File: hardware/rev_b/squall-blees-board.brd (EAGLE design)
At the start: 25.4 x 21 mm, 12 parts, among them J1 SQUALL_HEADER, J4 HIROSE-DF40C-10DP-0.4V, J5 HIROSE-DF40C-10DP-0.4V

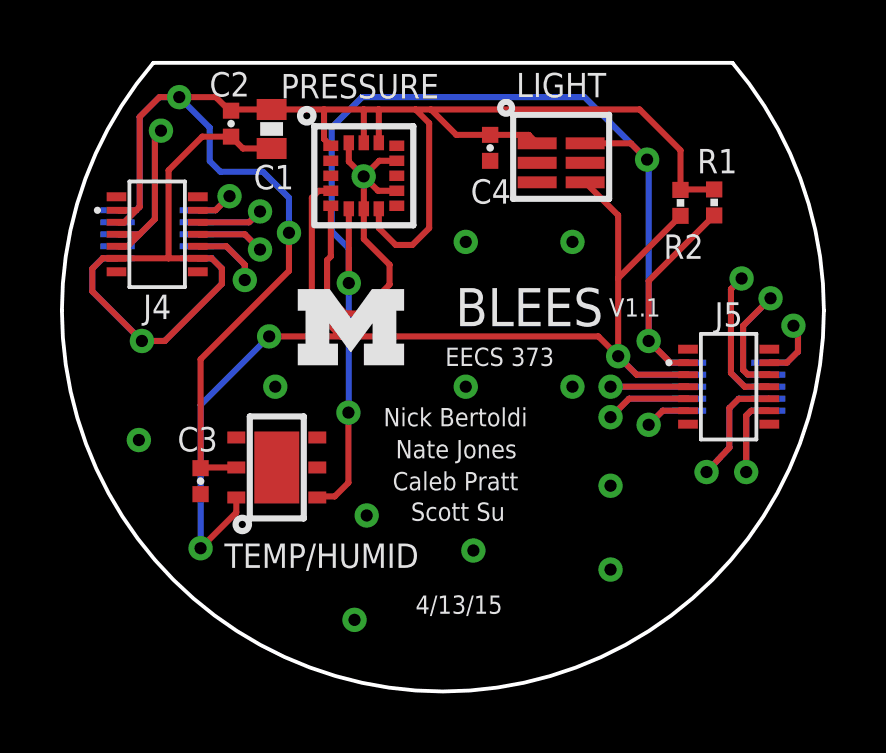
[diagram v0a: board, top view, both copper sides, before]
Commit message: Update rev_b, send it for fabrication
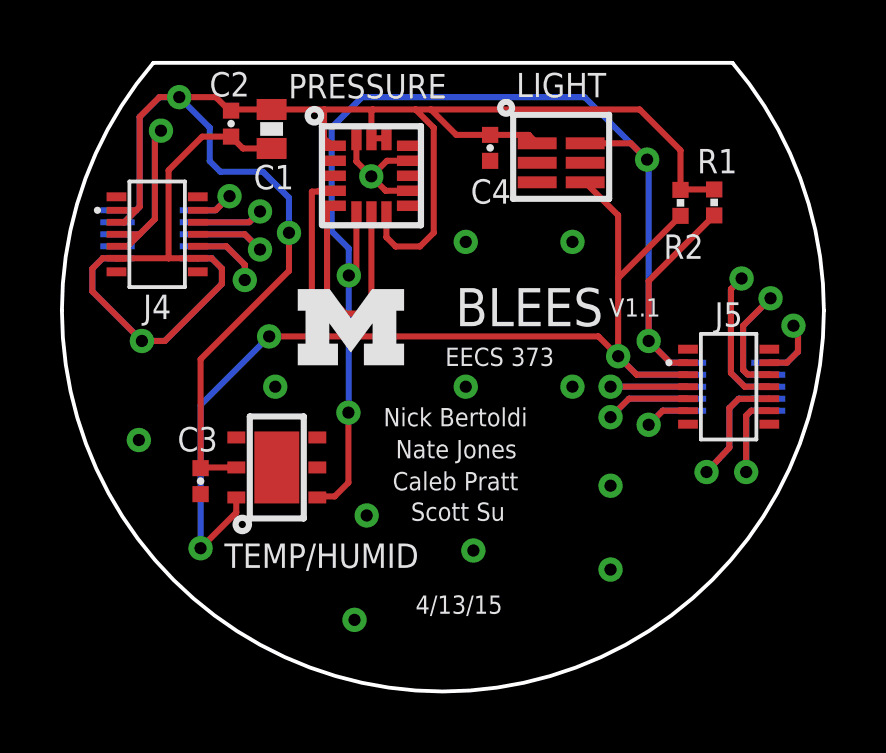
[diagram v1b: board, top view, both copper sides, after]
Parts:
- moved PRESSURE 0.25 mm to (21.7, 17.2)
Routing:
- net GND: track 41.4 -> 40.1 mm
- net VCC: track 63.9 -> 63.4 mm
